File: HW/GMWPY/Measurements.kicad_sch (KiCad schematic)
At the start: 35 parts, among them Q1 Q_PJFET_DSG, U10 LM4040DBZ-2.0, U3 USEQGCDACH4100, U4 TSV991ILT, U5 TSV991ILT, U6 EC4-1000-H2, U7 TSV991ILT, U8 TSV991ILT, U9 TSV991ILT

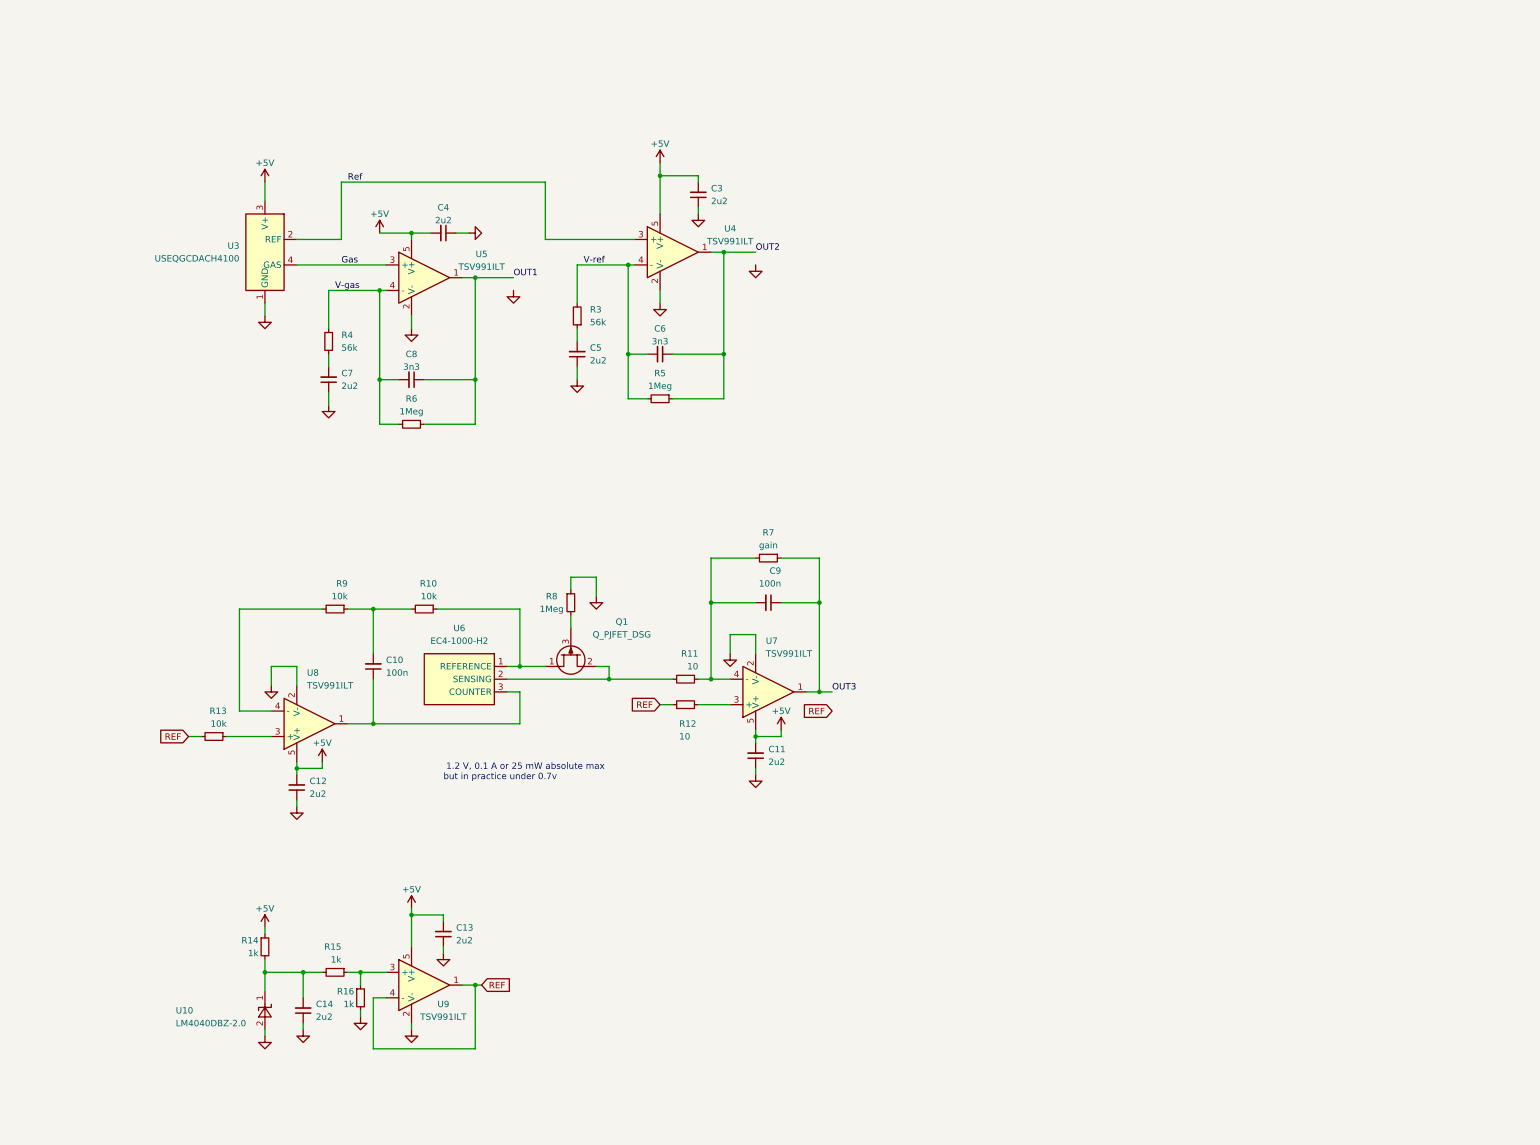
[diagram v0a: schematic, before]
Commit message: t
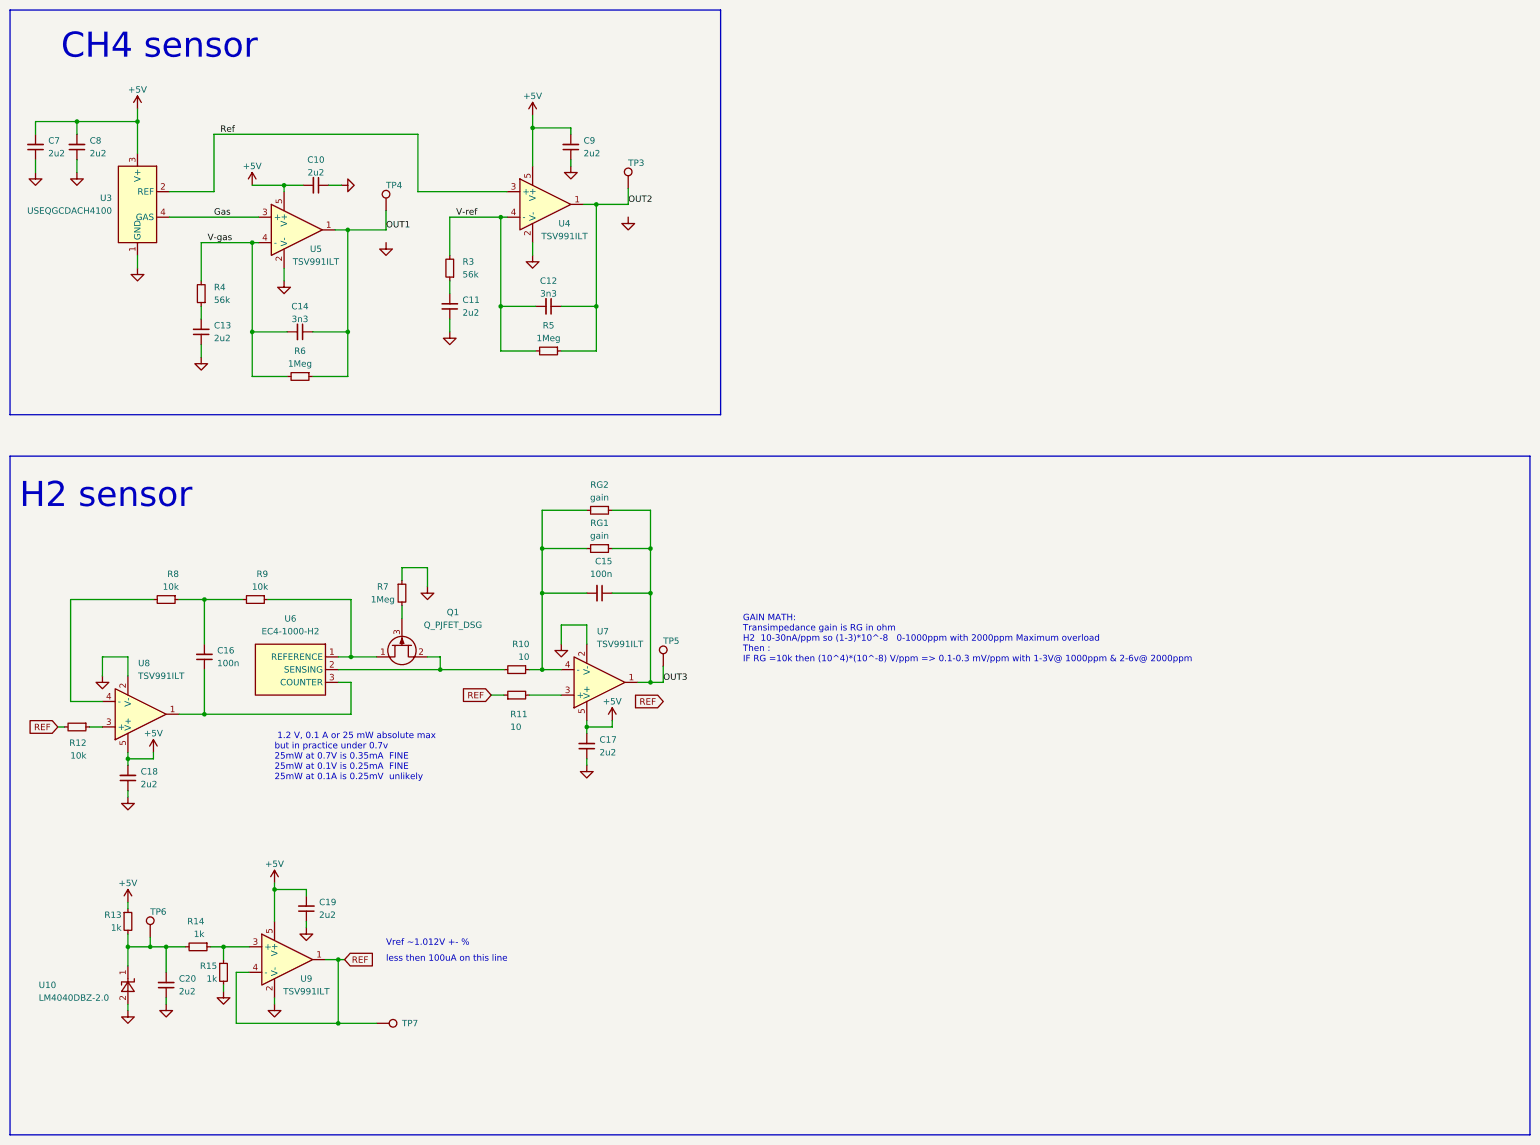
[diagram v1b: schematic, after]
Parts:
- added C7, C8: 2u2, Capacitor_SMD:C_0603_1608Metric, symbol Device:C_Small
- added RG2: gain, Resistor_SMD:R_0603_1608Metric, symbol Device:R_Small
- added TP3, TP4, TP5, TP6, TP7: TestPoint, TestPoint:TestPoint_THTPad_2.0x2.0mm_Drill1.0mm, symbol Connector:TestPoint
- renumbered C4 to C10, C5 to C11, C6 to C12, C7 to C13, C8 to C14, C9 to C15, C10 to C16, C11 to C17, C12 to C18, C13 to C19, C14 to C20, C3 to C9, R11 to R10, R12 to R11, R13 to R12, R14 to R13, R15 to R14, R16 to R15, R8 to R7, R9 to R8, R10 to R9, R7 to RG1
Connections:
- net +5V: now also C7.2, C8.2
- net GND: now also C7.1, C8.1
- net OUT1: now also TP4.1
- net OUT2: now also TP3.1
- net OUT3: now also RG2.1, TP5.1
- net REF: now also TP7.1
- net at C20.2, R13.2, R14.2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: now also TP6.1
- net at C15.2, R10.1, RG1.2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: now also RG2.2
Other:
- note added: "1.2 V, 0.1 A or 25 mW absolute max but in practice under 0.7v 25mW at 0.7V is 0.35mA FINE 25mW at 0.1V is 0.25mA FINE 25mW at 0.1A is 0.25mV unlikely"
- note added: "CH4 sensor"
- note added: "GAIN MATH: Transimpedance gain is RG in ohm H2 10-30nA/ppm so (1-3)*10^-8 0-1000ppm with 2000ppm Maximum overload Then : IF RG =10k then (10^4)*(10^-8) V/ppm => 0.1-0.3 mV/ppm with 1-3V@ 1000ppm & 2-6v@ 2000ppm"
- note added: "H2 sensor"
- note added: "Vref ~1.012V +- %"
- note added: "less then 100uA on this line"
- note removed: "1.2 V, 0.1 A or 25 mW absolute max but in practice under 0.7v"
- moved on the sheet: C10, C11, C12, C13, C14, C15, C16, C17, C18, C19, C20, C9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
